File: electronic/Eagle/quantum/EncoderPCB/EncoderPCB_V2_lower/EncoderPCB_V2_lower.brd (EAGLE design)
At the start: 150 x 30 mm, 20 parts, among them IC1 STM32F031K6T6

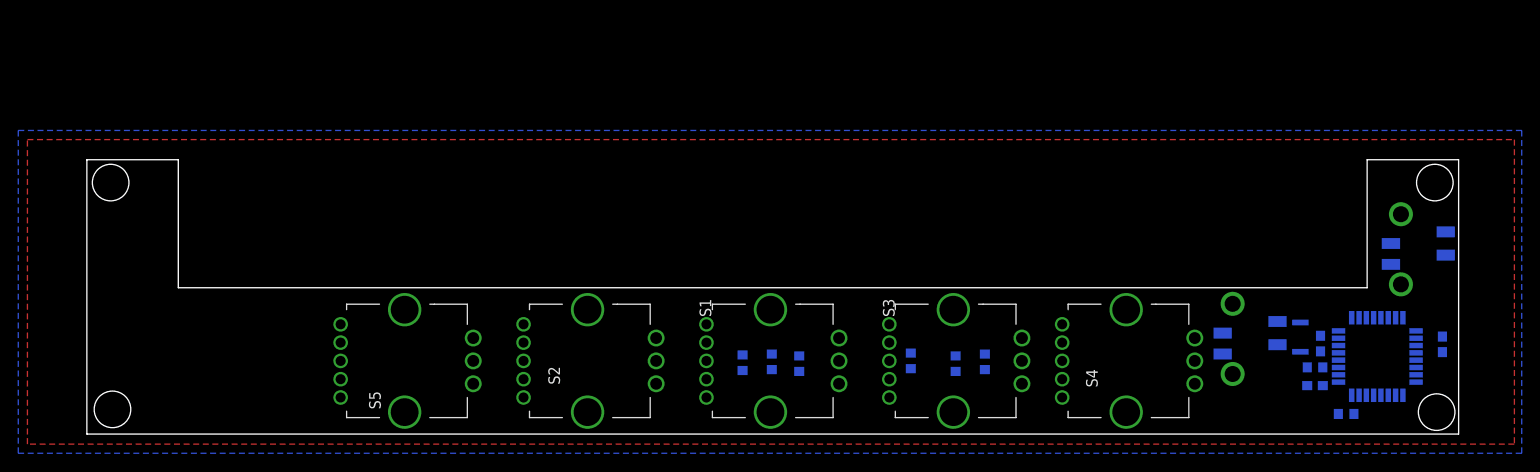
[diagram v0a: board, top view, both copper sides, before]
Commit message: progress on parametricEQ
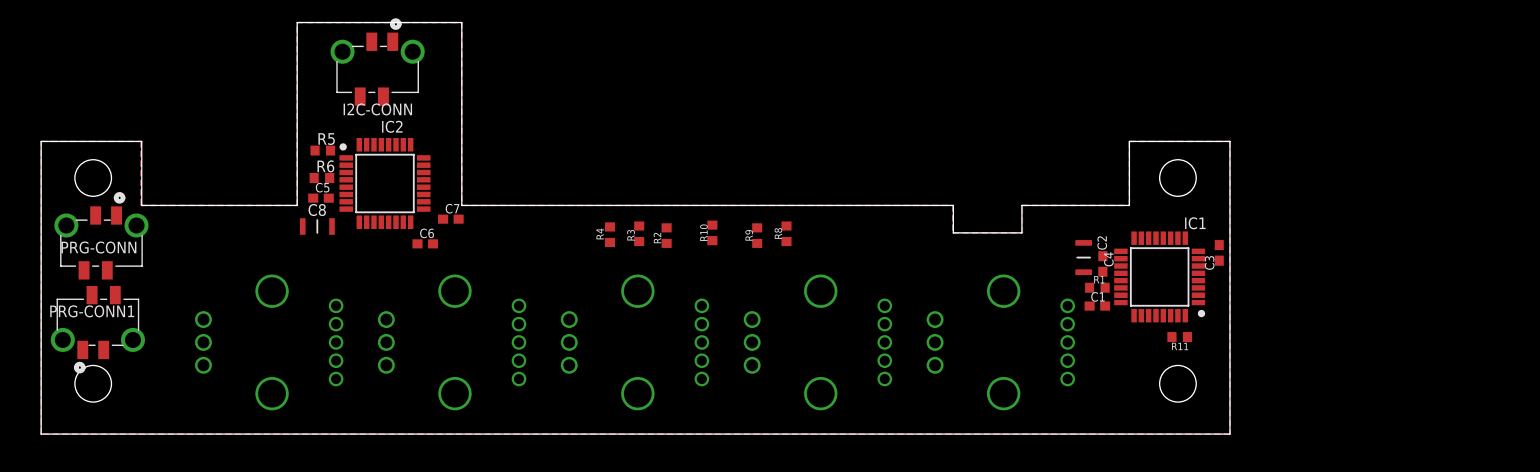
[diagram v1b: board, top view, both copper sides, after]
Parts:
- added C5, C6, C7: 100nF, C_Sager_Bibliothek:C0603
- added C8: 10 uF, passive components:C1206
- added IC2: STM32F031K6T6, C_Sager_Bibliothek:QFP80P900X900X160-32N
- added PRG-CONN1: 90814-0204, electro_mechanical:MOLEX_90814-0204
- added R5, R6: 10k, passive components:R0603
- moved PRG-CONN 139.2 mm to (8.50, 23.9), flipped to the top, turned to 180 degrees
- moved I2C-CONN 96.8 mm to (38.7, 42.9), flipped to the top, turned to 180 degrees
- moved C3 26.4 mm to (128.8, 19.8), flipped to the top
- moved R8 25.8 mm to (81.5, 21.9), flipped to the top
- moved R9 25.8 mm to (78.3, 21.7), flipped to the top
- moved R10 25.8 mm to (73.4, 22.0), flipped to the top
- moved C1 25.3 mm to (115.5, 14.0), flipped to the top
- moved C2 25.3 mm to (116.1, 18.6), flipped to the top
- moved IC1 25.3 mm to (122.3, 17.2), flipped to the top
- moved R1 25.3 mm to (115.5, 16.0), flipped to the top
- moved C4 25.2 mm to (114.0, 19.3), flipped to the top
- moved R2 20.2 mm to (68.4, 21.7), flipped to the top
- moved R4 20.2 mm to (62.2, 21.8), flipped to the top
- moved R3 20.2 mm to (65.4, 21.9), flipped to the top
- moved R11 20.0 mm to (124.5, 10.6), flipped to the top
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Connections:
- net +3V3: now also C5.1, C6.1, C7.1, C8.1, IC2.1, IC2.17, IC2.5
- net ADRR.: now also IC2.3, R5.2
- net BOOT_0: now also IC2.31, R6.2
- net BUTTON_ENC1: now also IC2.28
- net BUTTON_ENC2: now also IC2.30
- net BUTTON_ENC3: now also IC2.2
- net B_ENC1: now also IC2.11
- net B_ENC2: now also IC2.14
- net B_ENC3: now also IC2.27
- net ENCODER1_A: now also IC2.18
- net ENCODER1_B: now also IC2.19
- net ENCODER2_A: now also IC2.6
- net ENCODER2_B: now also IC2.7
- net ENCODER3_A: now also IC2.12
- net ENCODER3_B: now also IC2.13
- net GND: now also C5.2, C6.2, C7.2, C8.2, IC2.16, IC2.32, PRG-CONN1.4, R5.1, R6.1
- net G_ENC1: now also IC2.10
- net G_ENC2: now also IC2.22
- net G_ENC3: now also IC2.26
- net I2C1_SCL: now also IC2.29
- net I2C1_SDA: now also IC2.20
- net NRST: now also IC2.4, PRG-CONN1.2
- net R_ENC1: now also IC2.9
- net R_ENC2: now also IC2.21
- net R_ENC3: now also IC2.15
- net SWCLK: now also IC2.24, PRG-CONN1.1
- net SWDIO: now also IC2.23, PRG-CONN1.3
- net USART1_RX1: now also IC2.25
- net USART1_TX: now also IC2.8
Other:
- board size 150 x 30 mm -> 130 x 45 mm
